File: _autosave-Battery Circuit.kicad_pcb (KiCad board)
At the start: 2 copper layers, 36.4 x 39.7 mm, 43 parts, among them J1 1827685-4, J2 Programming Header (SWD), Q1 Si2309DS, Q2 BC847, SW1 SW_Push, U1 TPS54202DDC, U2 STM32G071KBUxN

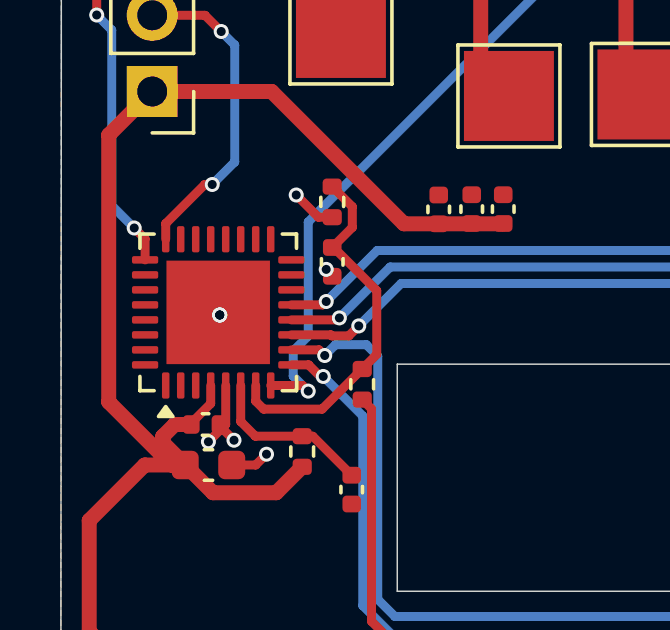
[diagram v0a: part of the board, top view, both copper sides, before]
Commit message: Fixed the warning
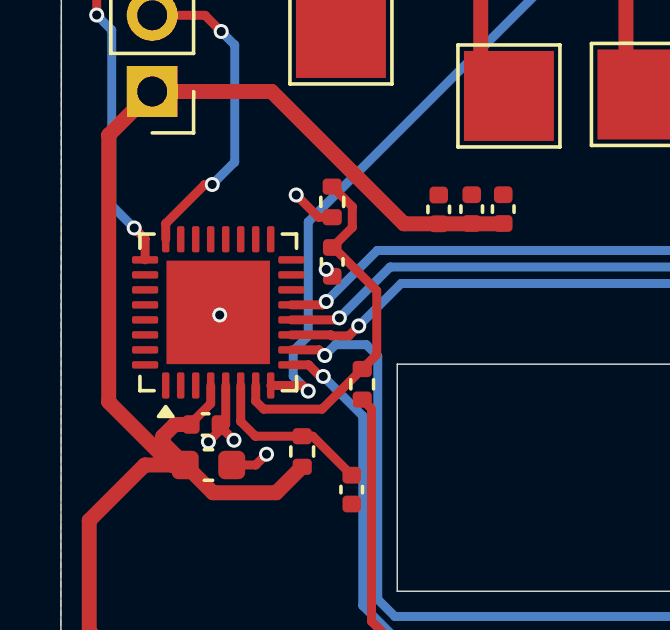
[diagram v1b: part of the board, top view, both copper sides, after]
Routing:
- net GND: vias 16 -> 15
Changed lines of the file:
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@@
-	)
-	(via
-		(at 133.1 76.75)
-		(size 0.5)
-		(drill 0.3)
-		(layers "F.Cu" "B.Cu")
-		(net "GND")
 	)
 	(via
